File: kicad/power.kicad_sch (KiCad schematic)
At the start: 13 parts, among them J12 Barrel_Jack, U4 TPS62142, U5 LP5907MFX-3.0

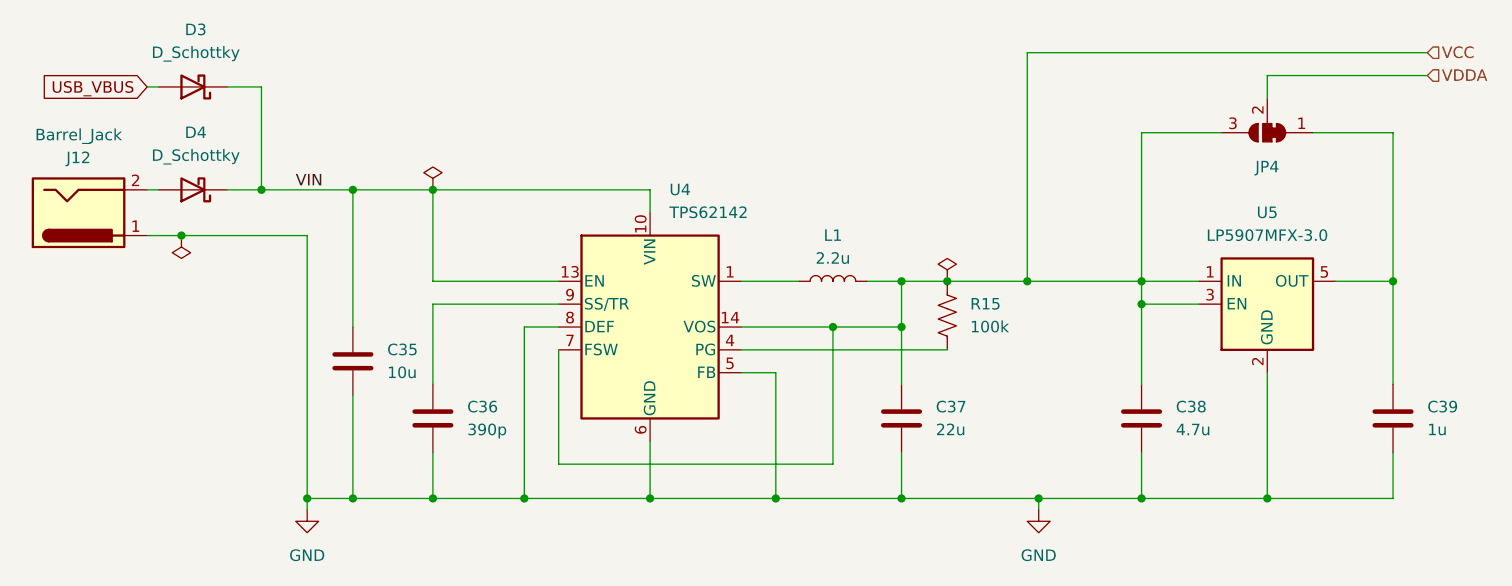
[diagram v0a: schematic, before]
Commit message: Add more parts
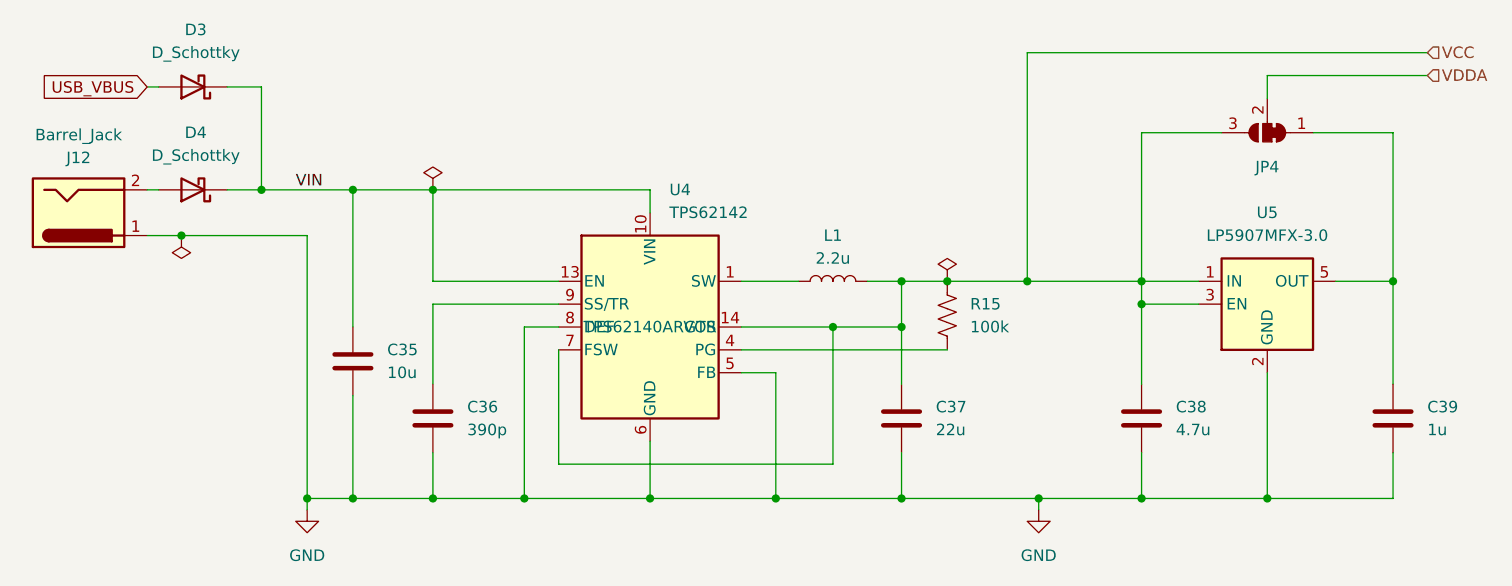
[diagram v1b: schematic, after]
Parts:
- U4: Part TPS62152RGTR -> TPS62140ARGTR
- U5: Part (none) -> LP5907MFX-3.0
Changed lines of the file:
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@@
+	)
+	(symbol
+		(lib_id "Regulator_Switching:TPS62142")
+		(at 134.62 104.14 0)
+		(unit 1)
+		(exclude_from_sim no)
+		(in_bom yes)
+		(on_board yes)
+		(dnp no)
+		(fields_autoplaced yes)
+		(property "Reference" "U4"
+			(at 136.7633 88.9 0)
+			(effects
+				(font
+					(size 1.27 1.27)
+				)
+				(justify left)
+			)
+		)
+		(property "Value" "TPS62142"
+			(at 136.7633 91.44 0)
+			(effects
+				(font
+					(size 1.27 1.27)
+				)
+				(justify left)
+			)
+		)
+		(property "Footprint" "Package_DFN_QFN:VQFN-16-1EP_3x3mm_P0.5mm_EP1.68x1.68mm_ThermalVias"
+			(at 138.43 115.57 0)
+			(effects
+				(font
+					(size 1.27 1.27)
+				)
+				(justify left)
+				(hide yes)
+			)
+		)
+		(property "Datasheet" "https://www.ti.com/lit/ds/symlink/tps62140.pdf"
+			(at 134.62 104.14 0)
+			(effects
+				(font
+					(size 1.27 1.27)
+				)
+				(hide yes)
+			)
+		)
+		(property "Description" "2A Step-Down Converter with DCS-Control, Fixed 3.3V Output Voltage, 3-17V Input Voltage, QFN-16"
+			(at 134.62 104.14 0)
+			(effects
+				(font
+					(size 1.27 1.27)
+				)
+				(hide yes)
+			)
+		)
+		(property "Part" "TPS62140ARGTR"
+			(at 134.62 104.14 0)
+			(effects
+				(font
+					(size 1.27 1.27)
+				)
+			)
+		)
+		(pin "17"
+		)
+		(pin "3"
+		)
+		(pin "15"
+		)
+		(pin "2"
+		)
+		(pin "13"
+		)
+		(pin "4"
+		)
+		(pin "5"
+		)
+		(pin "6"
+		)
+		(pin "1"
+		)
+		(pin "9"
+		)
+		(pin "8"
+		)
+		(pin "16"
+		)
+		(pin "7"
+		)
+		(pin "10"
+		)
+		(pin "11"
+		)
+		(pin "12"
+		)
+		(pin "14"
+		)
+		(instances
+			(project ""
+				(path "/79bfec23-3e7b-4837-8996-6bbe67be3d6b/50d1ea01-1e05-4a9c-ae07-2b1d5c2735d5"
+					(reference "U4")
+					(unit 1)
+				)
+			)
+		)
 	)
 	(symbol
@@
 			)
 		)
-		(property "Datasheet" "http://www.ti.com/lit/ds/symlink/lp5907.pdf"
+		(property "Datasheet" "https://www.ti.com/lit/ds/symlink/lp5907.pdf?ts=1771413737187"
 			(at 203.2 88.9 0)
 			(effects
@@
 		)
 		(property "Description" "250-mA Ultra-Low-Noise Low-IQ LDO, 3.0V, SOT-23"
+			(at 203.2 101.6 0)
+			(effects
+				(font
+					(size 1.27 1.27)
+				)
+				(hide yes)
+			)
+		)
+		(property "Part" "LP5907MFX-3.0"
 			(at 203.2 101.6 0)
 			(effects
@@
 					(unit 1)
 				)
-			)
-		)
-	)
-	(symbol
-		(lib_id "Regulator_Switching:TPS62142")
-		(at 134.62 104.14 0)
-		(unit 1)
-		(exclude_from_sim no)
-		(in_bom yes)
-		(on_board yes)
-		(dnp no)
-		(fields_autoplaced yes)
-		(property "Reference" "U4"
-			(at 136.7633 88.9 0)
-			(effects
-				(font
-					(size 1.27 1.27)
-				)
-				(justify left)
-			)
-		)
-		(property "Value" "TPS62142"
-			(at 136.7633 91.44 0)
-			(effects
-				(font
-					(size 1.27 1.27)
-				)
-				(justify left)
-			)
-		)
-		(property "Footprint" "Package_DFN_QFN:VQFN-16-1EP_3x3mm_P0.5mm_EP1.68x1.68mm_ThermalVias"
-			(at 138.43 115.57 0)
-			(effects
-				(font
-					(size 1.27 1.27)
-				)
-				(justify left)
-				(hide yes)
-			)
-		)
-		(property "Datasheet" "https://www.ti.com/lit/ds/symlink/tps62140.pdf?ts=1771407972175"
-			(at 134.62 104.14 0)
-			(effects
-				(font
-					(size 1.27 1.27)
-				)
-				(hide yes)
-			)
-		)
-		(property "Description" "2A Step-Down Converter with DCS-Control, Fixed 3.3V Output Voltage, 3-17V Input Voltage, QFN-16"
-			(at 134.62 104.14 0)
-			(effects
-				(font
-					(size 1.27 1.27)
-				)
-				(hide yes)
-			)
-		)
-		(property "Part" "TPS62152RGTR"
-			(at 134.62 104.14 0)
-			(effects
-				(font
-					(size 1.27 1.27)
-				)
-				(hide yes)
-			)
-		)
-		(pin "14"
-		)
-		(pin "16"
-		)
-		(pin "13"
-		)
-		(pin "9"
-		)
-		(pin "8"
-		)
-		(pin "1"
-		)
-		(pin "7"
-		)
-		(pin "6"
-		)
-		(pin "10"
-		)
-		(pin "11"
-		)
-		(pin "15"
-		)
-		(pin "4"
-		)
-		(pin "3"
-		)
-		(pin "17"
-		)
-		(pin "5"
-		)
-		(pin "2"
-		)
-		(pin "12"
-		)
-		(instances
-			(project "power"
-				(path "/04e31104-ef48-40c7-aa44-fb0b2d37d06e"
-					(reference "U?")
-					(unit 1)
-				)
-			)
-			(project "effect-pedal"
-				(path "/79bfec23-3e7b-4837-8996-6bbe67be3d6b/50d1ea01-1e05-4a9c-ae07-2b1d5c2735d5"
-					(reference "U4")
-					(unit 1)
-				)
